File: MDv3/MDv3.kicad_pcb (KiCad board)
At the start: 2 copper layers, 41 parts, among them J1 Conn_01x04_Pin, J3 XT60-M, J4 XT60-M

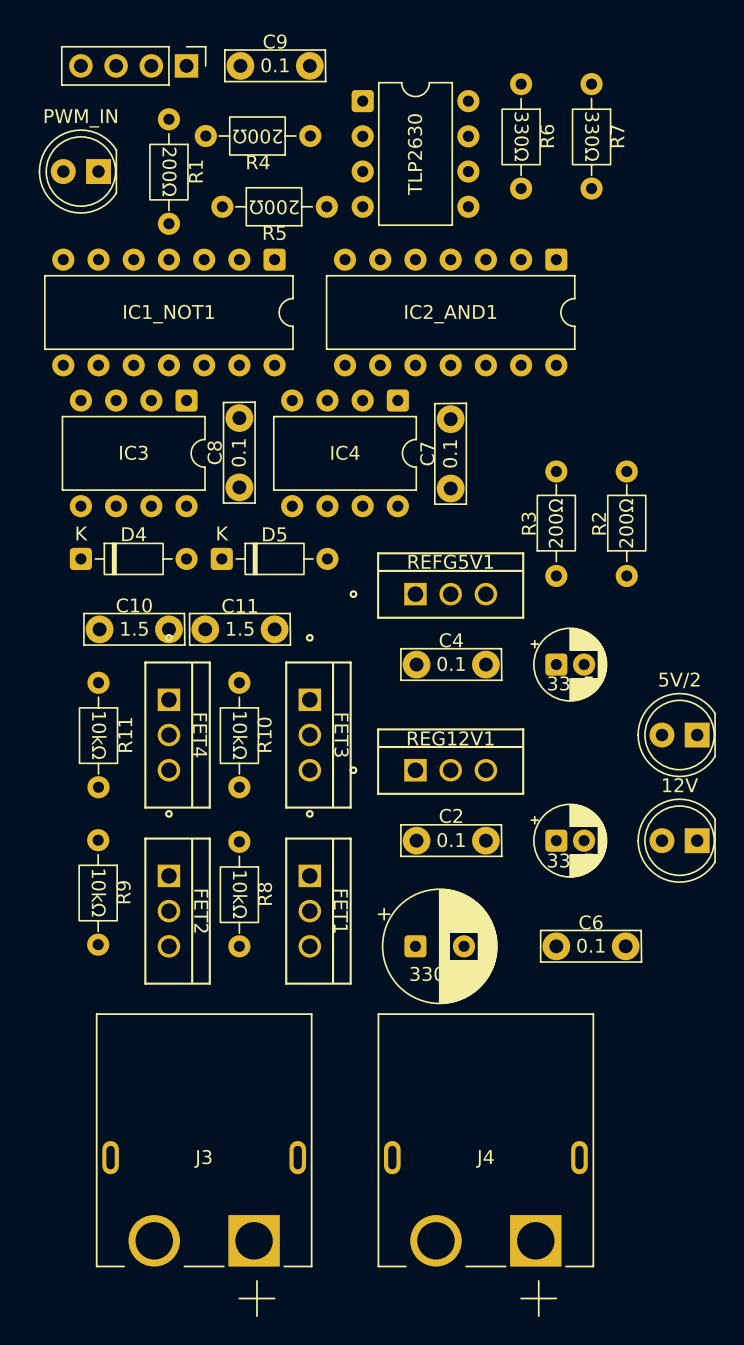
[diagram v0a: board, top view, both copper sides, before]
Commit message: 詰めた、配線する
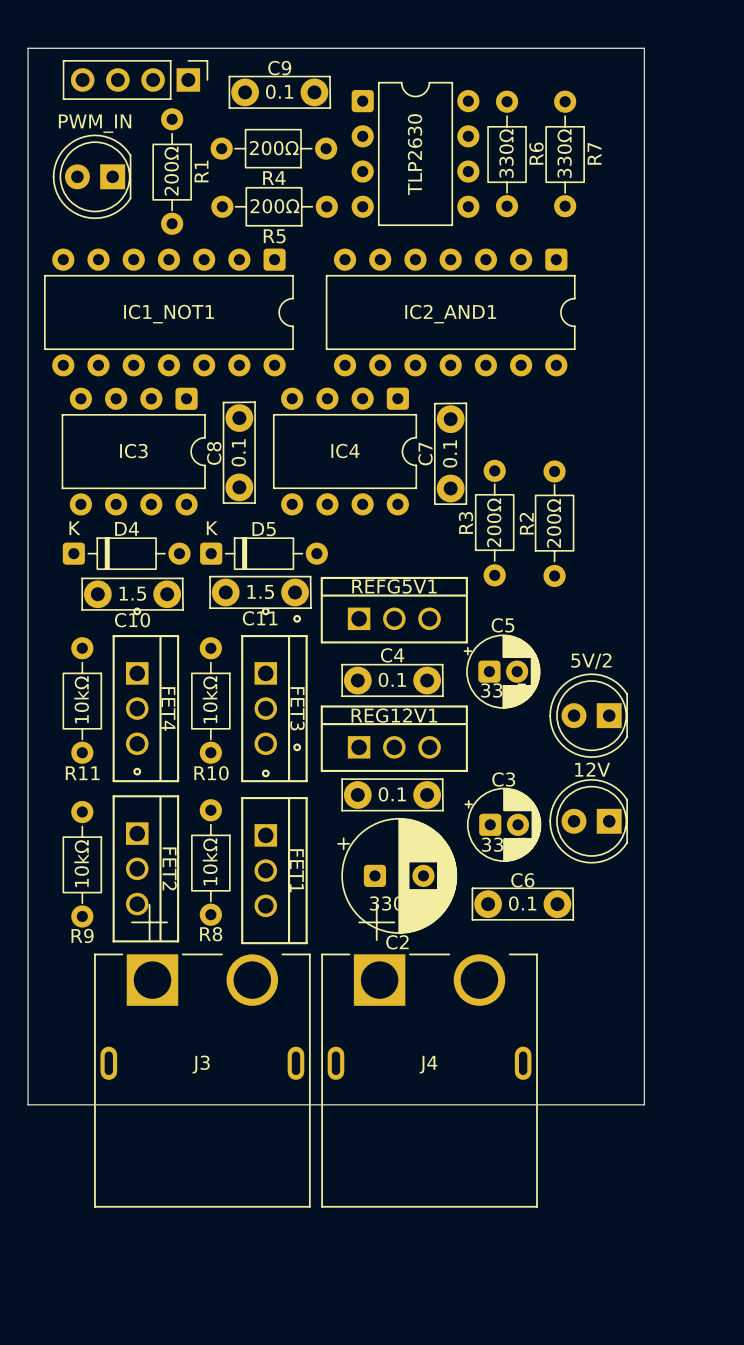
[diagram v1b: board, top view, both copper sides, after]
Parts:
- moved J4 7.93 mm to (128.0, 148.1), turned to 180 degrees
- moved J3 6.81 mm to (111.6, 148.1), turned to 180 degrees
- moved D3 6.50 mm to (141.0, 130.7)
- moved D2 6.50 mm to (141.0, 123.1)
- moved C1 5.86 mm to (124.1, 134.6)
- moved C6 5.78 mm to (132.2, 136.6)
- moved C2 5.37 mm to (122.8, 128.7)
- moved R2 5.21 mm to (137.0, 113.0)
- moved C3 4.90 mm to (132.4, 130.9)
- moved C5 4.85 mm to (132.3, 119.9)
- moved R3 4.45 mm to (132.7, 112.9)
- moved REFG5V1 4.44 mm to (122.9, 116.1)
- moved C4 4.39 mm to (122.8, 120.5)
- moved REG12V1 4.39 mm to (122.9, 125.3)
- moved FET1 4.31 mm to (116.2, 131.7)
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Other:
- board outline added: 44.4 x 76.2 mm
